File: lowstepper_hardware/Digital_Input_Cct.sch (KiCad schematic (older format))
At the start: 5 parts, among them J12 PJ398SM-12, Q1 MMBT3904

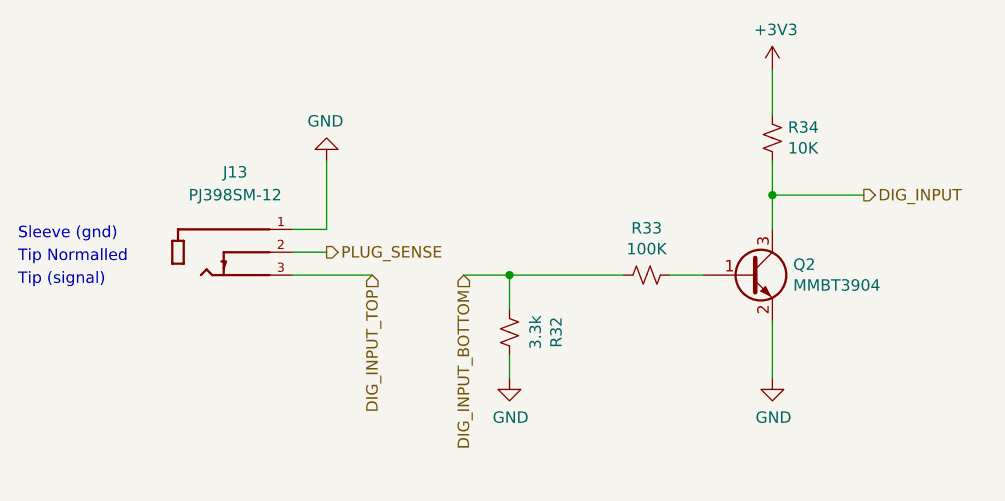
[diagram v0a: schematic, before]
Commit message: dancers hw
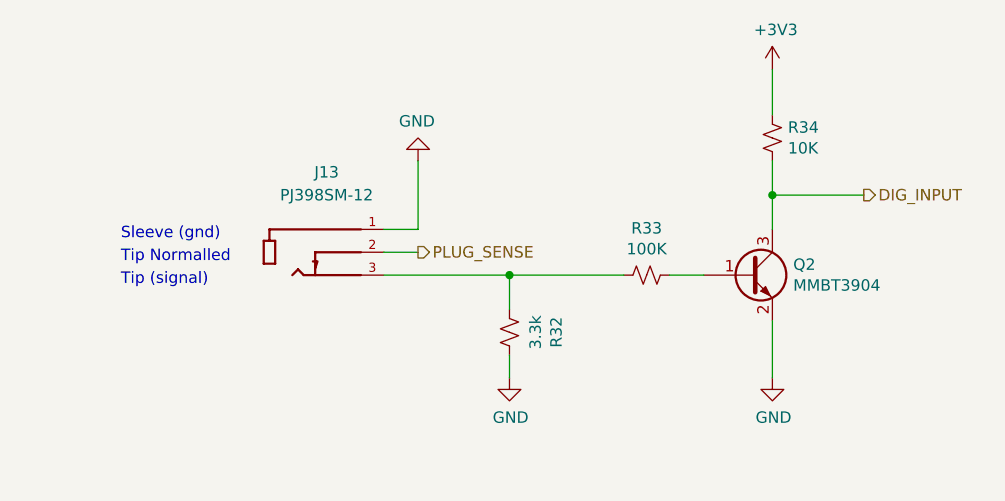
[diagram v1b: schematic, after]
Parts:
- R1, R4, R7: footprint Resistor_SMD:R_0603_1608Metric_Pad0.98x0.95mm_HandSolder -> Resistor_SMD:R_0402_1005Metric
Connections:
- net DIG_INPUT_TOP is gone; now on an unnamed net: J12.3
- net DIG_INPUT_BOTTOM: no longer names the net of R1.2, R4.2
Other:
- moved on the sheet: J13
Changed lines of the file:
@@
 $Descr A4 11693 8268
 encoding utf-8
-Sheet 13 13
+Sheet 5 8
 Title "Lowstepper"
 Date "2021-03-06"
@@
 F 0 "R32" V 5145 4000 50  0000 C CNN
 F 1 "3.3k" V 5236 4000 50  0000 C CNN
-F 2 "Resistor_SMD:R_0603_1608Metric_Pad0.98x0.95mm_HandSolder" H 5350 4000 50  0001 C CNN
+F 2 "Resistor_SMD:R_0402_1005Metric" H 5350 4000 50  0001 C CNN
 F 3 "~" H 5350 4000 50  0001 C CNN
 	1    5350 4000
@@
 F 0 "R34" H 6432 3104 50  0000 R CNN
 F 1 "10K" H 6432 3195 50  0000 R CNN
-F 2 "Resistor_SMD:R_0603_1608Metric_Pad0.98x0.95mm_HandSolder" H 6500 3150 50  0001 C CNN
+F 2 "Resistor_SMD:R_0402_1005Metric" H 6500 3150 50  0001 C CNN
 F 3 "~" H 6500 3150 50  0001 C CNN
 	1    6500 3150
@@
 Wire Wire Line
 	6500 3950 6500 4200
-$Comp
-L Device:R_Small_US R4
-U 1 1 60450238
-P 5950 3750
-AR Path="/6044C60B/60450238" Ref="R4"  Part="1"
-AR Path="/60488A39/60450238" Ref="R33"  Part="1"
-AR Path="/604956D4/60450238" Ref="R36"  Part="1"
-AR Path="/604A299D/60450238" Ref="R39"  Part="1"
-AR Path="/604B0276/60450238" Ref="R42"  Part="1"
-AR Path="/604BE180/60450238" Ref="R45"  Part="1"
-F 0 "R33" V 5745 3750 50  0000 C CNN
-F 1 "100K" V 5836 3750 50  0000 C CNN
-F 2 "Resistor_SMD:R_0603_1608Metric_Pad0.98x0.95mm_HandSolder" H 5950 3750 50  0001 C CNN
-F 3 "~" H 5950 3750 50  0001 C CNN
-	1    5950 3750
-	0    1    1    0
-$EndComp
 $Comp
 L power:GND #PWR0128
@@
 	1    0    0    -1
 $EndComp
-Text Notes 3200 3600 0    50   ~ 0
+Text Notes 3650 3600 0    50   ~ 0
 Sleeve (gnd)
-Text Notes 3200 3800 0    50   ~ 0
+Text Notes 3650 3800 0    50   ~ 0
 Tip (signal)
-Text Notes 3200 3700 0    50   ~ 0
+Text Notes 3650 3700 0    50   ~ 0
 Tip Normalled
-Wire Wire Line
-	4400 3750 4750 3750
-Wire Wire Line
-	4400 3550 4550 3550
-Wire Wire Line
-	4400 3650 4550 3650
-Text HLabel 4550 3650 2    50   Output ~ 0
-PLUG_SENSE
+Connection ~ 5350 3750
+$Comp
+L PJ398SM-12:PJ398SM-12 J12
+U 1 1 60450260
+P 4500 3550
+AR Path="/6044C60B/60450260" Ref="J12"  Part="1"
+AR Path="/60488A39/60450260" Ref="J13"  Part="1"
+AR Path="/604956D4/60450260" Ref="J14"  Part="1"
+AR Path="/604A299D/60450260" Ref="J15"  Part="1"
+AR Path="/604B0276/60450260" Ref="J16"  Part="1"
+AR Path="/604BE180/60450260" Ref="J17"  Part="1"
+F 0 "J13" H 4550 3800 50  0000 C CNN
+F 1 "PJ398SM-12" H 4550 3700 50  0000 C CNN
+F 2 "THONK_PJ398SM-12" H 4500 3550 50  0001 L BNN
+F 3 "" H 4500 3550 50  0001 L BNN
+F 4 "14.5 mm" H 4500 3550 50  0001 L BNN "MAXIMUM_PACKAGE_HEIGHT"
+F 5 "Thonk" H 4500 3550 50  0001 L BNN "MANUFACTURER"
+F 6 "1" H 4500 3550 50  0001 L BNN "PARTREV"
+F 7 "Manufacturer Recommendations" H 4500 3550 50  0001 L BNN "STANDARD"
+	1    4500 3550
+	1    0    0    -1
+$EndComp
+Wire Wire Line
+	4950 3550 4950 3250
 $Comp
 L power:GND #PWR0130
 U 1 1 60450250
-P 4550 3250
+P 4950 3250
 AR Path="/6044C60B/60450250" Ref="#PWR0130"  Part="1"
 AR Path="/60488A39/60450250" Ref="#PWR0149"  Part="1"
@@
 AR Path="/604B0276/60450250" Ref="#PWR0161"  Part="1"
 AR Path="/604BE180/60450250" Ref="#PWR0165"  Part="1"
-F 0 "#PWR0149" H 4550 3000 50  0001 C CNN
-F 1 "GND" H 4555 3077 50  0000 C CNN
-F 2 "" H 4550 3250 50  0001 C CNN
-F 3 "" H 4550 3250 50  0001 C CNN
-	1    4550 3250
+F 0 "#PWR0149" H 4950 3000 50  0001 C CNN
+F 1 "GND" H 4955 3077 50  0000 C CNN
+F 2 "" H 4950 3250 50  0001 C CNN
+F 3 "" H 4950 3250 50  0001 C CNN
+	1    4950 3250
 	-1   0    0    1
 $EndComp
-Wire Wire Line
-	4550 3550 4550 3250
-$Comp
-L PJ398SM-12:PJ398SM-12 J12
-U 1 1 60450260
-P 4100 3550
-AR Path="/6044C60B/60450260" Ref="J12"  Part="1"
-AR Path="/60488A39/60450260" Ref="J13"  Part="1"
-AR Path="/604956D4/60450260" Ref="J14"  Part="1"
-AR Path="/604A299D/60450260" Ref="J15"  Part="1"
-AR Path="/604B0276/60450260" Ref="J16"  Part="1"
-AR Path="/604BE180/60450260" Ref="J17"  Part="1"
-F 0 "J13" H 4150 3800 50  0000 C CNN
-F 1 "PJ398SM-12" H 4150 3700 50  0000 C CNN
-F 2 "THONK_PJ398SM-12" H 4100 3550 50  0001 L BNN
-F 3 "" H 4100 3550 50  0001 L BNN
-F 4 "14.5 mm" H 4100 3550 50  0001 L BNN "MAXIMUM_PACKAGE_HEIGHT"
-F 5 "Thonk" H 4100 3550 50  0001 L BNN "MANUFACTURER"
-F 6 "1" H 4100 3550 50  0001 L BNN "PARTREV"
-F 7 "Manufacturer Recommendations" H 4100 3550 50  0001 L BNN "STANDARD"
-	1    4100 3550
-	1    0    0    -1
-$EndComp
-Text HLabel 4750 3750 3    50   Input ~ 0
-DIG_INPUT_TOP
-Wire Wire Line
-	5350 3750 5150 3750
-Connection ~ 5350 3750
-Text HLabel 5150 3750 3    50   Input ~ 0
-DIG_INPUT_BOTTOM
+Text HLabel 4950 3650 2    50   Output ~ 0
+PLUG_SENSE
+Wire Wire Line
+	4800 3650 4950 3650
+Wire Wire Line
+	4800 3550 4950 3550
+Wire Wire Line
+	4800 3750 5350 3750
+$Comp
+L Device:R_Small_US R4
+U 1 1 60450238
+P 5950 3750
+AR Path="/6044C60B/60450238" Ref="R4"  Part="1"
+AR Path="/60488A39/60450238" Ref="R33"  Part="1"
+AR Path="/604956D4/60450238" Ref="R36"  Part="1"
+AR Path="/604A299D/60450238" Ref="R39"  Part="1"
+AR Path="/604B0276/60450238" Ref="R42"  Part="1"
+AR Path="/604BE180/60450238" Ref="R45"  Part="1"
+F 0 "R33" V 5745 3750 50  0000 C CNN
+F 1 "100K" V 5836 3750 50  0000 C CNN
+F 2 "Resistor_SMD:R_0402_1005Metric" H 5950 3750 50  0001 C CNN
+F 3 "~" H 5950 3750 50  0001 C CNN
+	1    5950 3750
+	0    1    1    0
+$EndComp
 $EndSCHEMATC
